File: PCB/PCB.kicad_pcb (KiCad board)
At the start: 2 copper layers, 91 x 76 mm, 20 parts, among them J1 Conn_01x03_Pin, J2 Conn_01x04_Pin, Q1 BC807, U1 Pico, U2 HX711

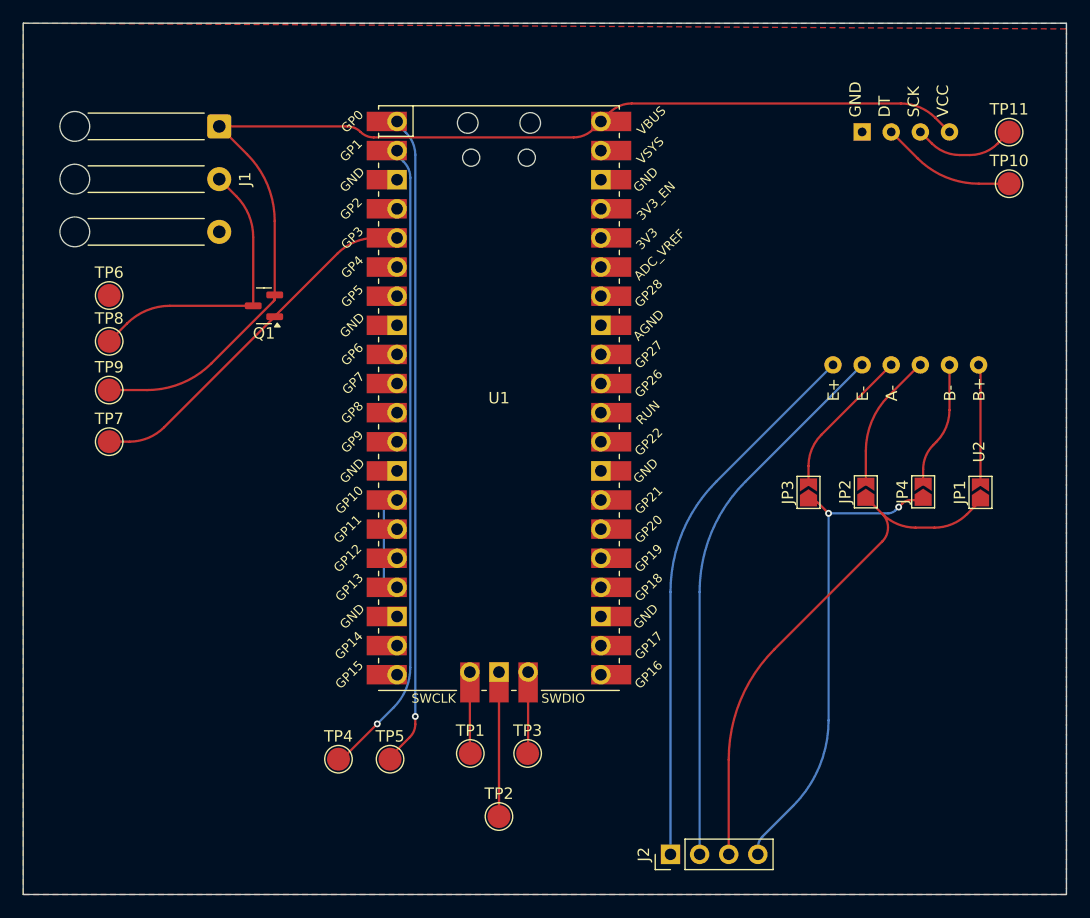
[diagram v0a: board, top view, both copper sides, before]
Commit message: schaltplan fertig
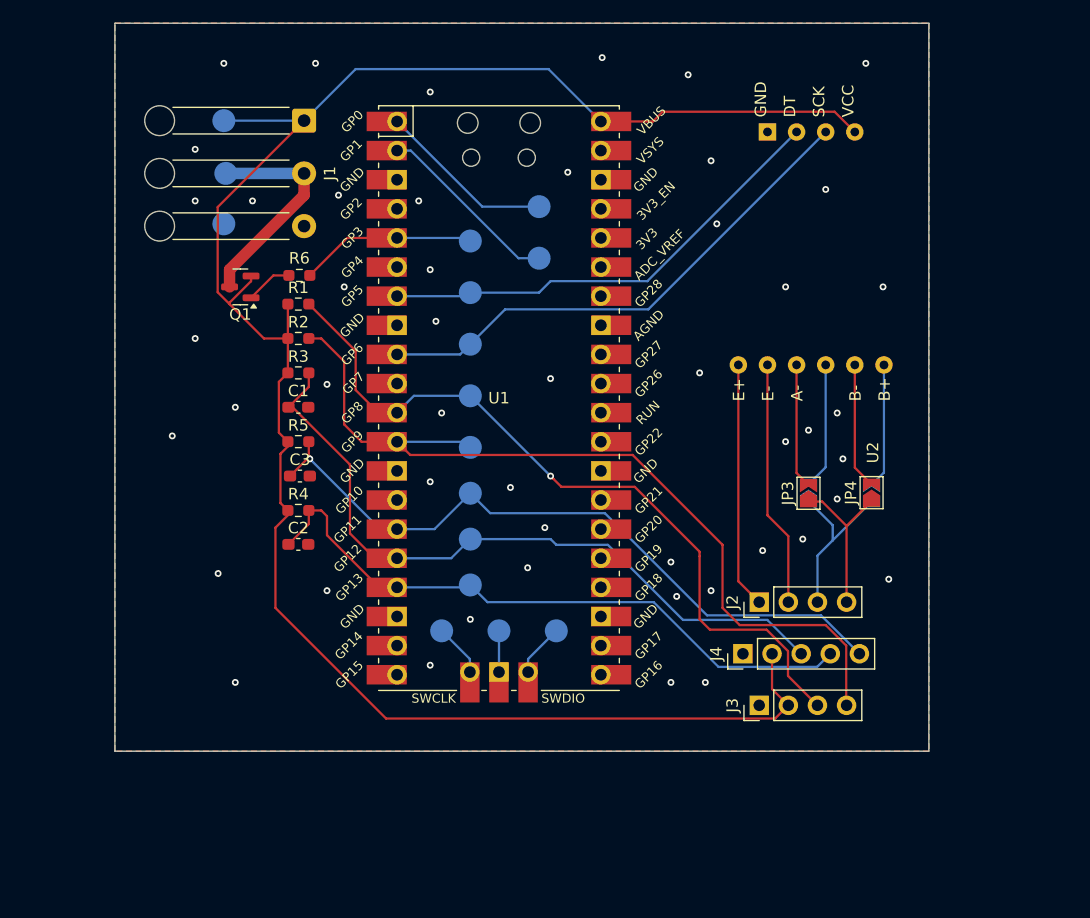
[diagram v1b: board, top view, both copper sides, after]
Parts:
- added C1: 100n, Capacitor_SMD:C_0603_1608Metric_Pad1.08x0.95mm_HandSolder, F.Cu at (91.5, 70.0)
- added C2: 100n, Capacitor_SMD:C_0603_1608Metric_Pad1.08x0.95mm_HandSolder, F.Cu at (91.5, 82.0)
- added C3: 100n, Capacitor_SMD:C_0603_1608Metric_Pad1.08x0.95mm_HandSolder, F.Cu at (91.6, 76.0)
- added J3: Conn_01x04_Socket, Connector_PinHeader_2.54mm:PinHeader_1x04_P2.54mm_Vertical, F.Cu at (131.7, 96.0)
- added J4: Conn_01x05_Socket, Connector_PinHeader_2.54mm:PinHeader_1x05_P2.54mm_Vertical, F.Cu at (130.3, 91.5)
- added R1: 3.3k, Resistor_SMD:R_0603_1608Metric_Pad0.98x0.95mm_HandSolder, F.Cu at (91.5, 61.0)
- added R2: 3.3k, Resistor_SMD:R_0603_1608Metric_Pad0.98x0.95mm_HandSolder, F.Cu at (91.5, 64.0)
- added R3: 3.3k, Resistor_SMD:R_0603_1608Metric_Pad0.98x0.95mm_HandSolder, F.Cu at (91.5, 67.0)
- added R4: 3.3k, Resistor_SMD:R_0603_1608Metric_Pad0.98x0.95mm_HandSolder, F.Cu at (91.5, 79.0)
- added R5: 3.3k, Resistor_SMD:R_0603_1608Metric_Pad0.98x0.95mm_HandSolder, F.Cu at (91.5, 73.0)
- added R6: 3.3k, Resistor_SMD:R_0603_1608Metric_Pad0.98x0.95mm_HandSolder, F.Cu at (91.6, 58.5)
- added TP12: TestPoint, TestPoint:TestPoint_Pad_D2.0mm, B.Cu at (106.5, 77.5)
- added TP13: TestPoint, TestPoint:TestPoint_Pad_D2.0mm, B.Cu at (106.5, 85.5)
- added TP14: TestPoint, TestPoint:TestPoint_Pad_D2.0mm, B.Cu at (106.5, 81.5)
- added TP15: TestPoint, TestPoint:TestPoint_Pad_D2.0mm, B.Cu at (106.5, 69.0)
- added TP16: TestPoint, TestPoint:TestPoint_Pad_D2.0mm, B.Cu at (106.5, 73.5)
- JP1, JP2, TP1, TP10, TP11, TP2, TP3, TP4, TP5, TP6, TP7, TP8, TP9: moved to B.Cu
- moved TP11 50.5 mm to (106.5, 64.5), turned to 180 degrees
- moved TP5 49.9 mm to (112.5, 52.5), turned to 180 degrees
- moved TP10 48.0 mm to (106.5, 60.0), turned to 180 degrees
- moved TP4 47.1 mm to (112.5, 57.0), turned to 180 degrees
- moved TP7 36.0 mm to (106.5, 55.5), turned to 180 degrees
- moved TP9 25.5 mm to (85.0, 45.0), turned to 180 degrees
- moved J2 23.3 mm to (131.7, 87.0)
- moved TP8 17.8 mm to (85.2, 49.6), turned to 180 degrees
- moved TP2 16.2 mm to (109.0, 89.5), turned to 180 degrees
- moved TP6 11.8 mm to (85.0, 54.0), turned to 180 degrees
- moved TP1 11.0 mm to (104.0, 89.5), turned to 180 degrees
- moved TP3 11.0 mm to (114.0, 89.5), turned to 180 degrees
- moved JP1 9.50 mm to (141.5, 77.5)
- moved U2 8.26 mm to (145.1, 73.9)
- moved J1 7.42 mm to (92.0, 45.0)
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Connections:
- TP7 pad 1: Net-(Q1-B) -> /Relay_3.3
- U1 pad 11: unconnected-(U1-GPIO8-Pad11) -> /LCD_SDA
- U1 pad 12: unconnected-(U1-GPIO9-Pad12) -> /LCD_SCL
- U1 pad 15: unconnected-(U1-GPIO11-Pad15) -> /encoder_button
- U1 pad 16: unconnected-(U1-GPIO12-Pad16) -> /encoder_a
- U1 pad 17: unconnected-(U1-GPIO13-Pad17) -> /encoder_b
- U1 pad 5: Net-(Q1-B) -> /Relay_3.3
- U1 pad 7: unconnected-(U1-GPIO5-Pad7) -> /HX/11_DT
- U1 pad 9: unconnected-(U1-GPIO6-Pad9) -> /HX711_SCK
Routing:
- net /LCD_SCL: track 0.00 -> 76.2 mm
- net +5V: track 100.2 -> 171.4 mm
- net /LCD_SDA: track 0.00 -> 67.2 mm, vias 0 -> 1
- net /encoder_a: track 0.00 -> 63.0 mm
- net /encoder_button: track 0.00 -> 61.6 mm, vias 0 -> 1
- net /encoder_b: track 0.00 -> 56.5 mm
- net Net-(U1-GPIO0): track 57.0 -> 15.5 mm, vias 1 -> 0
- net Net-(U1-GPIO1): track 56.0 -> 16.3 mm, vias 1 -> 0
- net /HX711_SCK: track 9.08 -> 45.4 mm
- net Net-(J2-Pin_3): track 46.4 -> 15.0 mm
- net Net-(J2-Pin_4): track 42.5 -> 13.9 mm, vias 2 -> 0
- net /HX/11_DT: track 12.3 -> 40.8 mm
- net Net-(Q1-B): track 32.1 -> 4.11 mm
- net Net-(J2-Pin_1): track 48.3 -> 21.4 mm
- net Net-(J2-Pin_2): track 47.9 -> 21.4 mm
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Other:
- board size 91 x 76 mm -> 71 x 63.5 mm
